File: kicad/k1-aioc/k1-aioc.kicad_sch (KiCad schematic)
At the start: 45 parts, among them J1 12401832E402A, J2 Conn_01x07_Male, Q1 BC847BS, U1 MIC5330-SSYML, U2 STM32F373CBTx, Y1 8MHz/20pF

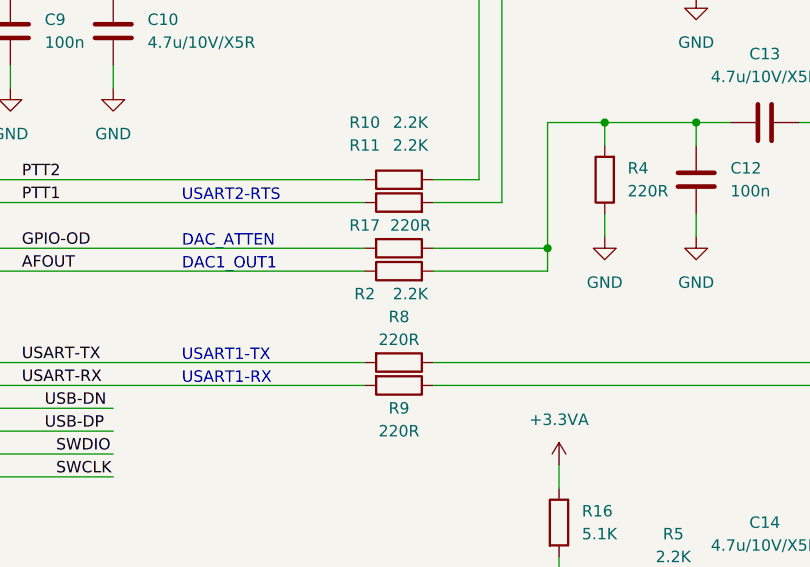
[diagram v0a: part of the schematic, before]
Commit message: Changed R2 to 5.1K to decrease DAC loading and reduce output level for radio microphone input
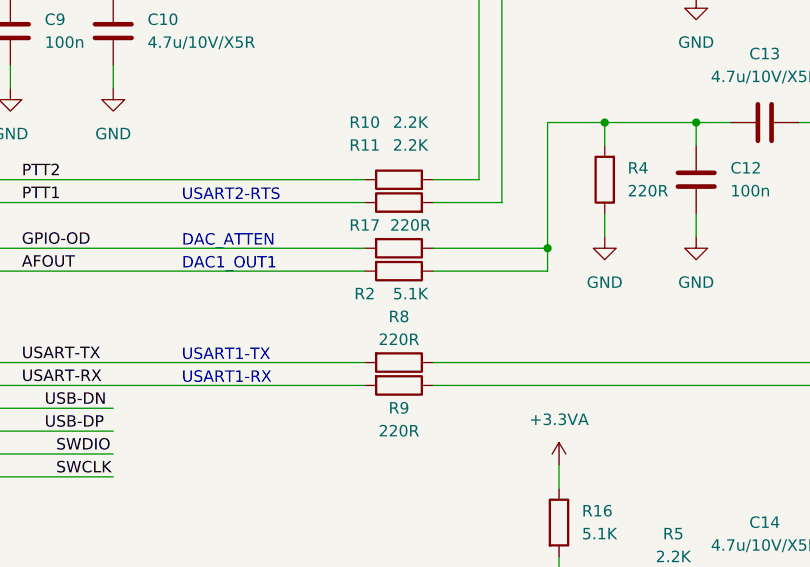
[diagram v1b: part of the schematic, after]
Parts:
- R2: value 2.2K -> 5.1K; LCSC C4190 -> C23186
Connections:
- net AFOUT: now also R2.2; no longer R2.1
- net at C12.1, C13.1, R17.1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: now also R2.1; no longer R2.2
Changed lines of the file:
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@@
     (pin "1")
-  )
-  (symbol (lib_id "Device:R") (at 184.15 106.68 90) (unit 1)
-    (in_bom yes) (on_board yes)
-    (property "Reference" "R2" (id 0) (at 180.34 109.22 90))
-    (property "Value" "2.2K" (id 1) (at 185.42 109.22 90))
-    (property "Footprint" "Resistor_SMD:R_0603_1608Metric" (id 2) (at 184.15 108.458 90)
-      (effects (font (size 1.27 1.27)) hide)
-    )
-    (property "Datasheet" "~" (id 3) (at 184.15 106.68 0)
-      (effects (font (size 1.27 1.27)) hide)
-    )
-    (property "LCSC" "C4190" (id 4) (at 180.34 109.22 0)
-      (effects (font (size 1.27 1.27)) hide)
-    )
-    (pin "1")
-    (pin "2")
   )
   (symbol (lib_id "Device:R") (at 232.41 36.83 270) (unit 1)
@@
     )
     (pin "1")
+  )
+  (symbol (lib_id "Device:R") (at 184.15 106.68 270) (unit 1)
+    (in_bom yes) (on_board yes)
+    (property "Reference" "R2" (id 0) (at 180.34 109.22 90))
+    (property "Value" "5.1K" (id 1) (at 185.42 109.22 90))
+    (property "Footprint" "Resistor_SMD:R_0603_1608Metric" (id 2) (at 184.15 104.902 90)
+      (effects (font (size 1.27 1.27)) hide)
+    )
+    (property "Datasheet" "~" (id 3) (at 184.15 106.68 0)
+      (effects (font (size 1.27 1.27)) hide)
+    )
+    (property "LCSC" "C23186" (id 4) (at 182.8799 104.14 0)
+      (effects (font (size 1.27 1.27)) hide)
+    )
+    (pin "1")
+    (pin "2")
   )
   (symbol (lib_id "Device:R") (at 201.93 134.62 0) (unit 1)
@@
       (reference "R1") (unit 1) (value "1.5K") (footprint "Resistor_SMD:R_0603_1608Metric")
     )
-    (path "/5d94c761-144d-4672-9330-c6fa3412fb4e"
-      (reference "R2") (unit 1) (value "2.2K") (footprint "Resistor_SMD:R_0603_1608Metric")
+    (path "/a395a1f6-0ade-49ae-97ea-2e311cd442a3"
+      (reference "R2") (unit 1) (value "5.1K") (footprint "Resistor_SMD:R_0603_1608Metric")
     )
     (path "/a6e41ec9-f152-4bb3-b386-4a1ce2030945"
